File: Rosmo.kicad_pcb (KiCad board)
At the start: 2 copper layers, 88.4 x 99.3 mm, 106 parts, among them J1 C2904998, J2 C2904998, J3 C2904998, J4 C2904998, J5 CONN-SMD_4P-P1.00_SM04B-SRSS-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, P3 C2897365, P4 HDR-TH_2P-P2.54-V-F, U11 M3_STANDOFF, U12 M3_STANDOFF, U13 CONN-TH_DG308-2.54-02P-14-00A, U14 CONN-TH_DG308-2.54-02P-14-00A, U15 M3_STANDOFF, U16 C2718488, U17 M3_STANDOFF, U18 M3_STANDOFF, U19 M3_STANDOFF, U2 Pb, U20 N20-40MM-WHEEL, U21 N20-40MM-WHEEL, U22 RECTANGULAR_HOLE, U23 RECTANGULAR_HOLE, U24 N20-40MM-WHEEL, U25 M3_STANDOFF, U26 M3_STANDOFF, U28 CONN-TH_DB125-2.54-10P-GN, U29 RECTANGULAR_M3, U3 HDR-TH_6P-P2.54-H-F-W5.7, U30 RECTANGULAR_M3, U31 RECTANGULAR_M3, U32 RECTANGULAR_M3, U33 C2845567, U34 CONN-TH_DB125-2.54-10P-GN, U39 N20-40MM-WHEEL, U40 RECTANGULAR_M3, U41 RECTANGULAR_M3, U42 RECTANGULAR_M3, U43 RECTANGULAR_M3, U45 C2895059, U48 C2895059, U49 C2895059, U5 HDR-TH_22P-P2.54-V-F, U50 C2886702, U51 C2886702, U52 CONN-TH_DB125-2.54-10P-GN, U53 CONN-TH_DB125-2.54-10P-GN, U55 PWM, U6 C2895059, U7 C2886702, U8 RECTANGULAR_HOLE, U9 RECTANGULAR_HOLE

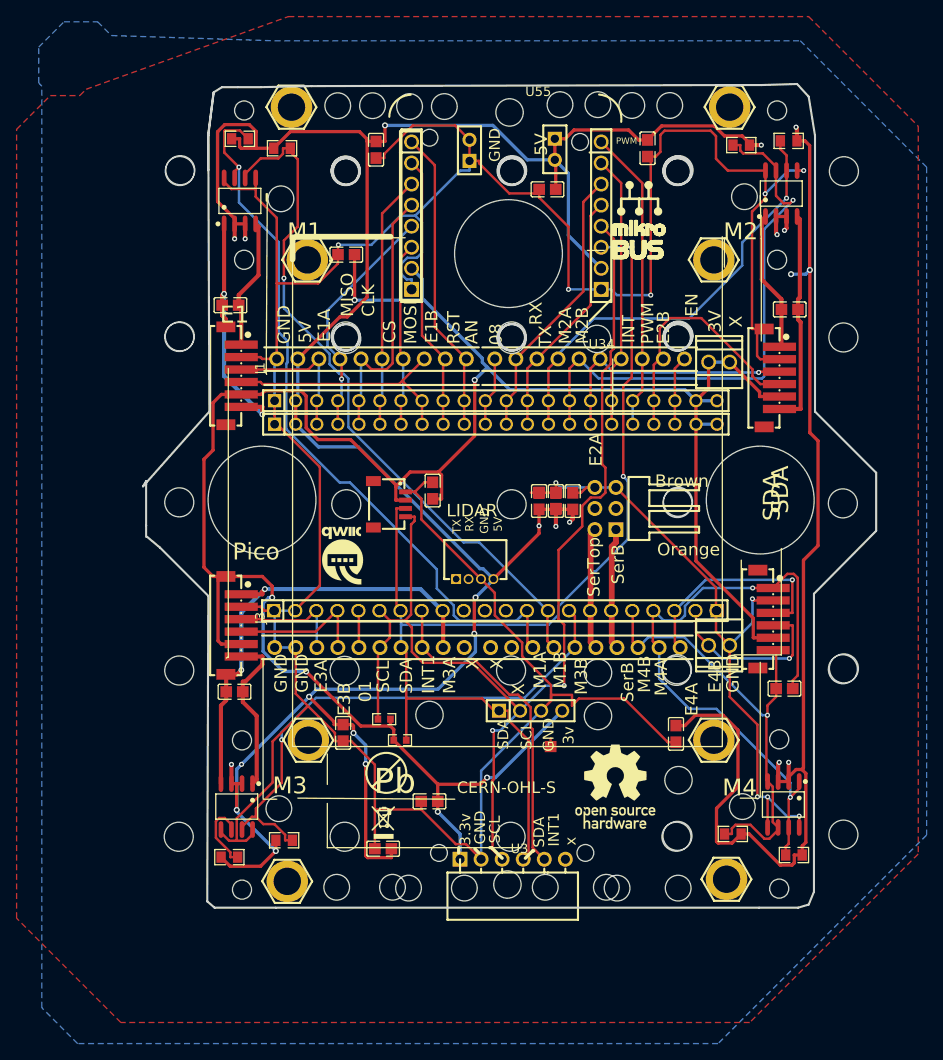
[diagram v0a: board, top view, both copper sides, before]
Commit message: Added JLPCB production files
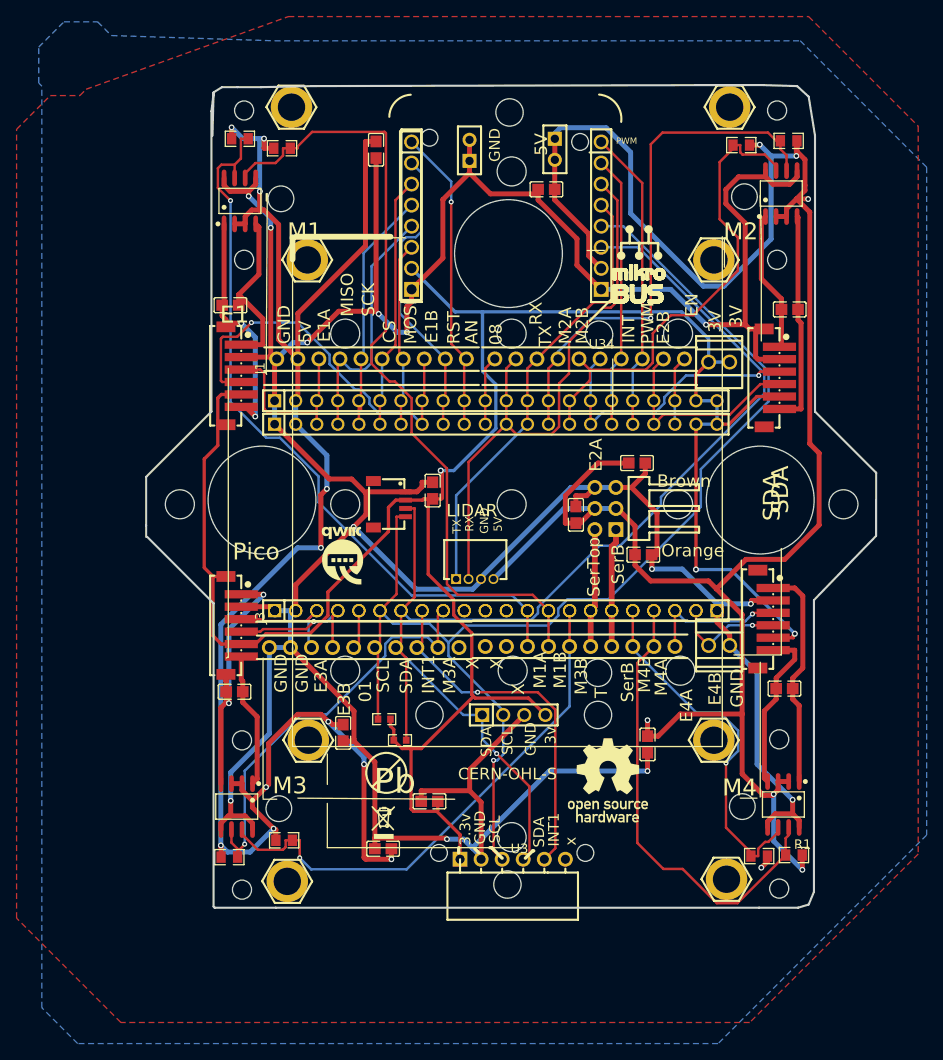
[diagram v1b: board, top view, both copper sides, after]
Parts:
- removed 20MM: ORP ORIGINAL 5X5 - NO EXTRA, easyeda:ORP ORIGINAL 5X5 - NO EXTRA
- removed the ? at (58.4, 21.3)
- removed the ? at (65.5, 48.3)
- removed the ? at (65.4, 2.79)
- removed the ? at (60.5, 21.3)
- removed the ? at (60.5, 23.2)
- removed the ? at (59.8, 51.9)
- removed the ? at (75.2, 56.0)
- removed C11, C13: C49678, easyeda:C0805
- removed R10: C17414, easyeda:R0805
- removed U29, U30, U31, U32, U40, U41, U42, U43: RECTANGULAR_M3, easyeda:RECTANGULAR_M3
- removed U55: PWM, easyeda:MIKROBUS_SILK
- added ?: , AutoGenerated:MountingHole_3.30mm, F.Cu at (65.7, 2.29)
- added ?: , AutoGenerated:MountingHole_3.30mm, F.Cu at (65.5, 48.1)
- added R1: C17414, easyeda:R0805, F.Cu at (89.2, 65.0)
- added U35: PWM, easyeda:MIKROBUS_SILK, F.Cu at (54.4, -12.1)
- added U38: ORP ROSMO - NO EXTRA, easyeda:ORP ROSMO - NO EXTRA, F.Cu at (65.7, 22.2)
- added U44: HOLECUT, easyeda:HOLECUT, F.Cu at (67.2, 68.8)
- added U46: HOLECUT, easyeda:HOLECUT, F.Cu at (42.2, 68.8)
- added U47: HOLECUT, easyeda:HOLECUT, F.Cu at (67.4, -25.3)
- added U54: HOLECUT, easyeda:HOLECUT, F.Cu at (41.3, -25.3)
- P4: value HDR-TH_2P-P2.54-V-F -> C49661
- U3: value HDR-TH_6P-P2.54-H-F-W5.7 -> C2833720
- moved C7 14.1 mm to (71.0, 28.8), turned to 180 degrees
- moved C6 10.8 mm to (70.2, 17.8), turned to 180 degrees
- moved R9 4.15 mm to (85.0, 65.2)
- moved C15 3.66 mm to (71.5, 51.7)
- moved U16 2.09 mm to (55.4, 48.1)
- moved C1 1.69 mm to (62.9, 24.0)
- moved .5 1.17 mm to (66.5, 55.4)
- moved U53 0.65 mm to (63.4, 39.9)
- moved U52 0.63 mm to (37.3, 40.0)
- moved U22 0.52 mm to (33.8, 55.1)
- moved U23 0.36 mm to (76.3, 55.1)
- moved U9 0.18 mm to (76.2, -20.6)
- moved C10 0.13 mm to (59.3, -15.2)
- moved U51 0.13 mm to (53.2, 35.6)
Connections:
- C5 pad 1: M4CB -> M4B
- C5 pad 2: M4CA -> M4A
- J1 pad 8: (no net) -> 3V
- J4 pad 1: M4CA -> M4A
- J4 pad 6: M4CB -> M4B
- U33 pad 1: S$352179 -> TX
- U33 pad 2: S$352450 -> RX
- U49 pad 1: M4CA -> M4A
- U49 pad 4: M4CB -> M4B
- U49 pad 7: M4CA -> MC4A
- U5 pad 14: M3A -> M3CA
- U5 pad 4: M4CA -> MC4A
- U51 pad 19: M4CA -> MC4A
- U51 pad 9: M3A -> M3CA
- U52 pad 2: M3A -> M3CA
- U53 pad 2: M4CA -> MC4A
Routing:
- net M4CA: track 75.6 -> 0.00 mm, vias 2 -> 0
- net MC4A: track 0.00 -> 55.6 mm
- net M3CA: track 8.89 -> 49.8 mm, vias 0 -> 1
- net RX: track 33.7 -> 69.7 mm
- net M4A: track 0.00 -> 27.2 mm
- net M3A: track 56.8 -> 31.8 mm
- net TX: track 30.1 -> 54.6 mm
- net M4B: track 0.00 -> 20.1 mm
- net E1B: track 29.6 -> 46.8 mm, vias 0 -> 1
- net SDA: track 133.4 -> 149.3 mm, vias 2 -> 1
- net SCL: track 137.4 -> 151.5 mm, vias 2 -> 1
- net M1CB: track 84.1 -> 97.4 mm, vias 1 -> 0
- net M4CB: track 56.2 -> 44.1 mm
- net M2CA: track 53.1 -> 63.8 mm
- net E4A: track 26.8 -> 17.1 mm
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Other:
- board size 88.4 x 99.3 mm -> 88 x 99.2 mm
- board text added: "SCK"
- board text added: "T"
- board text added: "Version 0.7"
- board text removed: "CLK"
- board text removed: "Version 0.5"
